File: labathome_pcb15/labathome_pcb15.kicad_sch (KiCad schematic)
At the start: 41 parts, among them J11 USB_ESP32, J15 CAN RS 485, J17 Micro_SD_Card_Det1, J21 GPIO, J22 Volts, J6 I2C, J7 PROG ESP, SW2 YELLOW, SW3 GREEN, SW3 Reset, SW4 RED, U2 ESP32-S3-WROOM-1, U21 IPS_240_240, U3 SRV05-4

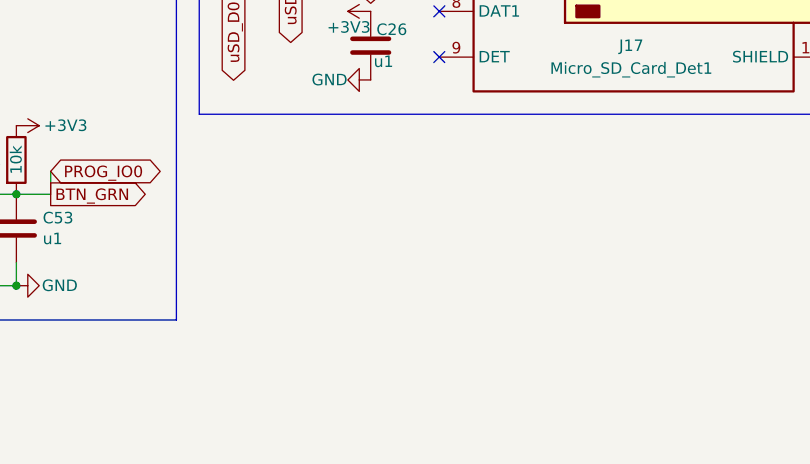
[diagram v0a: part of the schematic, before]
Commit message: bsec
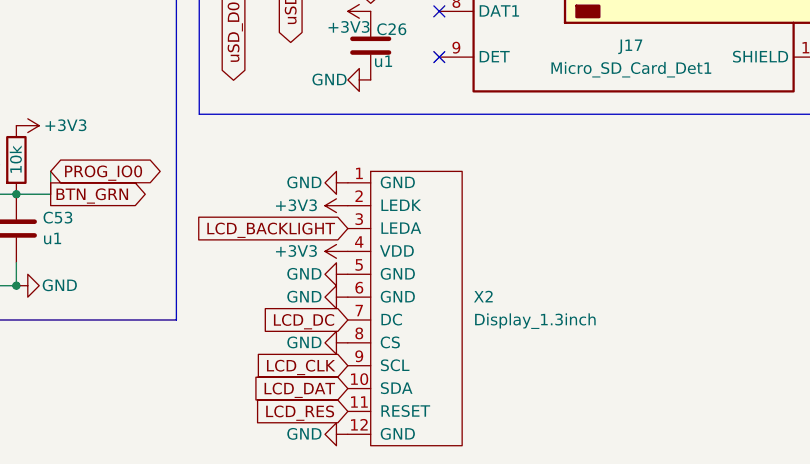
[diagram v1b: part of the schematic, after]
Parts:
- added X2: Display_1.3inch, liebler_OPTO:IPS_130, symbol liebler_OPTO:Display_LH154K-PG04
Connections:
- net +3V3: now also X2.2 (LEDK), X2.4 (VDD)
- net GND: now also X2.1 (GND), X2.12 (GND), X2.5 (GND), X2.6 (GND), X2.8 (CS)
- net LCD_BACKLIGHT: now also X2.3 (LEDA)
- net LCD_CLK: now also X2.9 (SCL)
- net LCD_DAT: now also X2.10 (SDA)
- net LCD_DC: now also X2.7 (DC)
- net LCD_RES: now also X2.11 (RESET)
